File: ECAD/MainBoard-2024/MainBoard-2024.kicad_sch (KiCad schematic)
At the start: 65 parts, among them J1 XT60, J10 Conn_01x02, J11 Conn_01x03, J12 Conn_01x04, J13 Conn_01x03, J14 Conn_01x03, J15 Conn_01x02, J16 XT30, J17 XT30, J18 Conn_01x02, J2 Conn_01x04, J20 BAU, J21 BAU, J22 Conn_01x04, J23 Conn_01x02, J26 BAU, J27 BAU, J28 Conn_01x02, J29 Conn_01x02, J3 ConStep1, J30 Conn_01x03, J4 Conn_01x02, J5 ConStep1, J6 ConStep1, J7 XT30, J8 Conn_01x02, J9 Conn_01x02, K2 FINDER-36.11, U1 Teensy3.5_All_Pins, U2 R-78B3.3-2.0, U3 R-78B12-2.0, U4 R-78B5.0-2.0

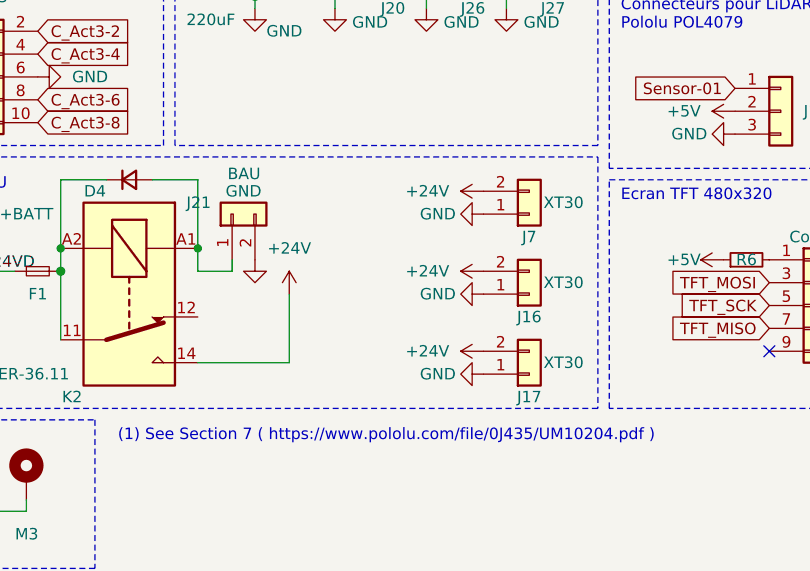
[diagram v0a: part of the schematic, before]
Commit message: Clean positions
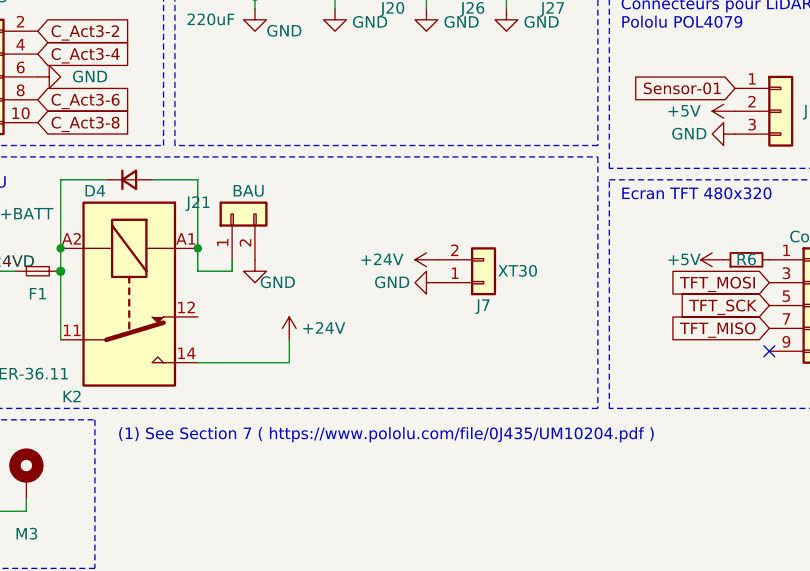
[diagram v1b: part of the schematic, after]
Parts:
- removed J16, J17: XT30, Connector_AMASS:AMASS_XT30U-F_1x02_P5.0mm_Vertical, symbol Connector_Generic:Conn_01x02
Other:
- moved on the sheet: J7
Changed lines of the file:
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@@
     (stroke (width 0) (type solid))
   )
-  (wire (pts (xy 196.85 152.4) (xy 196.85 160.02))
+  (wire (pts (xy 196.85 157.48) (xy 196.85 160.02))
     (stroke (width 0) (type default))
   )
@@
       (effects (font (size 1.27 1.27)) hide)
     )
-    (property "Value" "GND" (at 191.77 140.97 0)
+    (property "Value" "GND" (at 195.58 151.13 0)
       (effects (font (size 1.27 1.27)))
     )
@@
     )
   )
-  (symbol (lib_id "power:+24V") (at 196.85 152.4 0) (unit 1)
-    (in_bom yes) (on_board yes) (dnp no) (fields_autoplaced)
-    (property "Reference" "#PWR0157" (at 196.85 156.21 0)
+  (symbol (lib_id "power:+24V") (at 196.85 157.48 0) (unit 1)
+    (in_bom yes) (on_board yes) (dnp no)
+    (property "Reference" "#PWR0157" (at 196.85 161.29 0)
       (effects (font (size 1.27 1.27)) hide)
     )
-    (property "Value" "+24V" (at 196.85 147.32 0)
+    (property "Value" "+24V" (at 200.66 156.21 0)
       (effects (font (size 1.27 1.27)))
     )
-    (property "Footprint" "" (at 196.85 152.4 0)
+    (property "Footprint" "" (at 196.85 157.48 0)
       (effects (font (size 1.27 1.27)) hide)
     )
-    (property "Datasheet" "" (at 196.85 152.4 0)
+    (property "Datasheet" "" (at 196.85 157.48 0)
       (effects (font (size 1.27 1.27)) hide)
     )
@@
     )
   )
-  (symbol (lib_id "power:+24V") (at 218.44 140.97 90) (unit 1)
+  (symbol (lib_id "power:+24V") (at 213.36 148.59 90) (unit 1)
     (in_bom yes) (on_board yes) (dnp no) (fields_autoplaced)
-    (property "Reference" "#PWR0189" (at 222.25 140.97 0)
+    (property "Reference" "#PWR0189" (at 217.17 148.59 0)
       (effects (font (size 1.27 1.27)) hide)
     )
-    (property "Value" "+24V" (at 214.63 140.9699 90)
+    (property "Value" "+24V" (at 209.55 148.5899 90)
       (effects (font (size 1.27 1.27)) (justify left))
     )
-    (property "Footprint" "" (at 218.44 140.97 0)
+    (property "Footprint" "" (at 213.36 148.59 0)
       (effects (font (size 1.27 1.27)) hide)
     )
-    (property "Datasheet" "" (at 218.44 140.97 0)
+    (property "Datasheet" "" (at 213.36 148.59 0)
       (effects (font (size 1.27 1.27)) hide)
     )
@@
       (effects (font (size 1.27 1.27)) (justify right))
     )
-    (property "Value" "BAU" (at 189.9921 139.036 90)
+    (property "Value" "BAU" (at 190.5 140.97 90)
       (effects (font (size 1.27 1.27)) (justify right))
     )
@@
     )
   )
-  (symbol (lib_id "power:+24V") (at 218.44 158.75 90) (unit 1)
-    (in_bom yes) (on_board yes) (dnp no) (fields_autoplaced)
-    (property "Reference" "#PWR0185" (at 222.25 158.75 0)
-      (effects (font (size 1.27 1.27)) hide)
-    )
-    (property "Value" "+24V" (at 214.63 158.7499 90)
-      (effects (font (size 1.27 1.27)) (justify left))
-    )
-    (property "Footprint" "" (at 218.44 158.75 0)
-      (effects (font (size 1.27 1.27)) hide)
-    )
-    (property "Datasheet" "" (at 218.44 158.75 0)
-      (effects (font (size 1.27 1.27)) hide)
-    )
-    (pin "1")
-    (instances
-      (project "MainBoard-2024"
-        (path "/b1b0855c-c4b6-47dd-8ac8-2346963564b3"
-          (reference "#PWR0185") (unit 1)
-        )
-      )
-    )
-  )
   (symbol (lib_id "Regulator_Switching:R-78B5.0-2.0") (at 187.96 27.94 0) (unit 1)
     (in_bom yes) (on_board yes) (dnp no)
@@
     )
   )
-  (symbol (lib_id "power:GND") (at 218.44 161.29 270) (unit 1)
-    (in_bom yes) (on_board yes) (dnp no)
-    (property "Reference" "#PWR0187" (at 212.09 161.29 0)
-      (effects (font (size 1.27 1.27)) hide)
-    )
-    (property "Value" "GND" (at 213.36 161.29 90)
-      (effects (font (size 1.27 1.27)))
-    )
-    (property "Footprint" "" (at 218.44 161.29 0)
-      (effects (font (size 1.27 1.27)) hide)
-    )
-    (property "Datasheet" "" (at 218.44 161.29 0)
-      (effects (font (size 1.27 1.27)) hide)
-    )
-    (pin "1")
-    (instances
-      (project "MainBoard-2024"
-        (path "/b1b0855c-c4b6-47dd-8ac8-2346963564b3"
-          (reference "#PWR0187") (unit 1)
-        )
-      )
-    )
-  )
   (symbol (lib_id "power:+3V3") (at 262.89 148.59 270) (unit 1)
     (in_bom yes) (on_board yes) (dnp no) (fields_autoplaced)
@@
     )
   )
-  (symbol (lib_id "Connector_Generic:Conn_01x02") (at 223.52 161.29 0) (mirror x) (unit 1)
-    (in_bom yes) (on_board yes) (dnp no)
-    (property "Reference" "J17" (at 223.52 163.83 0)
-      (effects (font (size 1.27 1.27)))
-    )
-    (property "Value" "XT30" (at 227.33 160.02 0)
-      (effects (font (size 1.27 1.27)))
-    )
-    (property "Footprint" "Connector_AMASS:AMASS_XT30U-F_1x02_P5.0mm_Vertical" (at 223.52 161.29 0)
-      (effects (font (size 1.27 1.27)) hide)
-    )
-    (property "Datasheet" "~" (at 223.52 161.29 0)
-      (effects (font (size 1.27 1.27)) hide)
-    )
-    (pin "1")
-    (pin "2")
-    (instances
-      (project "MainBoard-2024"
-        (path "/b1b0855c-c4b6-47dd-8ac8-2346963564b3"
-          (reference "J17") (unit 1)
-        )
-      )
-    )
-  )
   (symbol (lib_id "Connector_Generic:Conn_01x04") (at 234.95 76.2 0) (mirror y) (unit 1)
     (in_bom yes) (on_board yes) (dnp no)
@@
     )
   )
-  (symbol (lib_id "power:GND") (at 218.44 152.4 270) (unit 1)
-    (in_bom yes) (on_board yes) (dnp no)
-    (property "Reference" "#PWR0186" (at 212.09 152.4 0)
-      (effects (font (size 1.27 1.27)) hide)
-    )
-    (property "Value" "GND" (at 213.36 152.4 90)
-      (effects (font (size 1.27 1.27)))
-    )
-    (property "Footprint" "" (at 218.44 152.4 0)
-      (effects (font (size 1.27 1.27)) hide)
-    )
-    (property "Datasheet" "" (at 218.44 152.4 0)
-      (effects (font (size 1.27 1.27)) hide)
-    )
-    (pin "1")
-    (instances
-      (project "MainBoard-2024"
-        (path "/b1b0855c-c4b6-47dd-8ac8-2346963564b3"
-          (reference "#PWR0186") (unit 1)
-        )
-      )
-    )
-  )
   (symbol (lib_id "Connector_Generic:Conn_01x02") (at 208.28 115.57 0) (unit 1)
     (in_bom yes) (on_board yes) (dnp no)
@@
     )
   )
-  (symbol (lib_id "power:+24V") (at 218.44 149.86 90) (unit 1)
-    (in_bom yes) (on_board yes) (dnp no) (fields_autoplaced)
-    (property "Reference" "#PWR0158" (at 222.25 149.86 0)
-      (effects (font (size 1.27 1.27)) hide)
-    )
-    (property "Value" "+24V" (at 214.63 149.8599 90)
-      (effects (font (size 1.27 1.27)) (justify left))
-    )
-    (property "Footprint" "" (at 218.44 149.86 0)
-      (effects (font (size 1.27 1.27)) hide)
-    )
-    (property "Datasheet" "" (at 218.44 149.86 0)
-      (effects (font (size 1.27 1.27)) hide)
-    )
-    (pin "1")
-    (instances
-      (project "MainBoard-2024"
-        (path "/b1b0855c-c4b6-47dd-8ac8-2346963564b3"
-          (reference "#PWR0158") (unit 1)
-        )
-      )
-    )
-  )
   (symbol (lib_id "power:GND") (at 46.99 45.72 270) (unit 1)
     (in_bom yes) (on_board yes) (dnp no) (fields_autoplaced)
@@
     )
   )
-  (symbol (lib_id "Connector_Generic:Conn_01x02") (at 223.52 143.51 0) (mirror x) (unit 1)
+  (symbol (lib_id "Connector_Generic:Conn_01x02") (at 218.44 151.13 0) (mirror x) (unit 1)
     (in_bom yes) (on_board yes) (dnp no)
-    (property "Reference" "J7" (at 223.52 146.05 0)
+    (property "Reference" "J7" (at 218.44 153.67 0)
       (effects (font (size 1.27 1.27)))
     )
-    (property "Value" "XT30" (at 227.33 142.24 0)
+    (property "Value" "XT30" (at 222.25 149.86 0)
       (effects (font (size 1.27 1.27)))
     )
-    (property "Footprint" "Connector_AMASS:AMASS_XT30U-F_1x02_P5.0mm_Vertical" (at 223.52 143.51 0)
+    (property "Footprint" "Connector_AMASS:AMASS_XT30U-F_1x02_P5.0mm_Vertical" (at 218.44 151.13 0)
       (effects (font (size 1.27 1.27)) hide)
     )
-    (property "Datasheet" "~" (at 223.52 143.51 0)
+    (property "Datasheet" "~" (at 218.44 151.13 0)
       (effects (font (size 1.27 1.27)) hide)
     )
@@
     )
   )
-  (symbol (lib_id "power:GND") (at 218.44 143.51 270) (unit 1)
+  (symbol (lib_id "power:GND") (at 213.36 151.13 270) (unit 1)
     (in_bom yes) (on_board yes) (dnp no)
-    (property "Reference" "#PWR0188" (at 212.09 143.51 0)
+    (property "Reference" "#PWR0188" (at 207.01 151.13 0)
       (effects (font (size 1.27 1.27)) hide)
     )
-    (property "Value" "GND" (at 213.36 143.51 90)
+    (property "Value" "GND" (at 208.28 151.13 90)
       (effects (font (size 1.27 1.27)))
     )
-    (property "Footprint" "" (at 218.44 143.51 0)
+    (property "Footprint" "" (at 213.36 151.13 0)
       (effects (font (size 1.27 1.27)) hide)
     )
-    (property "Datasheet" "" (at 218.44 143.51 0)
+    (property "Datasheet" "" (at 213.36 151.13 0)
       (effects (font (size 1.27 1.27)) hide)
     )
@@
         )
       )
-    )
-  )
-  (symbol (lib_id "Connector_Generic:Conn_01x02") (at 223.52 152.4 0) (mirror x) (unit 1)
-    (in_bom yes) (on_board yes) (dnp no)
-    (property "Reference" "J16" (at 223.52 154.94 0)
-      (effects (font (size 1.27 1.27)))
-    )
-    (property "Value" "XT30" (at 227.33 151.13 0)
-      (effects (font (size 1.27 1.27)))
-    )
-    (property "Footprint" "Connector_AMASS:AMASS_XT30U-F_1x02_P5.0mm_Vertical" (at 223.52 152.4 0)
-      (effects (font (size 1.27 1.27)) hide)
-    )
-    (property "Datasheet" "~" (at 223.52 152.4 0)
-      (effects (font (size 1.27 1.27)) hide)
-    )
-    (pin "1")
-    (pin "2")
-    (instances
-      (project "MainBoard-2024"
-        (path "/b1b0855c-c4b6-47dd-8ac8-2346963564b3"
-          (reference "J16") (unit 1)
-        )
-      )
